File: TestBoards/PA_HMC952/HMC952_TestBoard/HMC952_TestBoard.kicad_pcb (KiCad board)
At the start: 2 copper layers, 60 x 45 mm, 31 parts, among them J1 SMA, J2 SMA, J3 VDD, J4 VGG, J5 VDET, J6 VDET, U1 HMC952ALP5GE

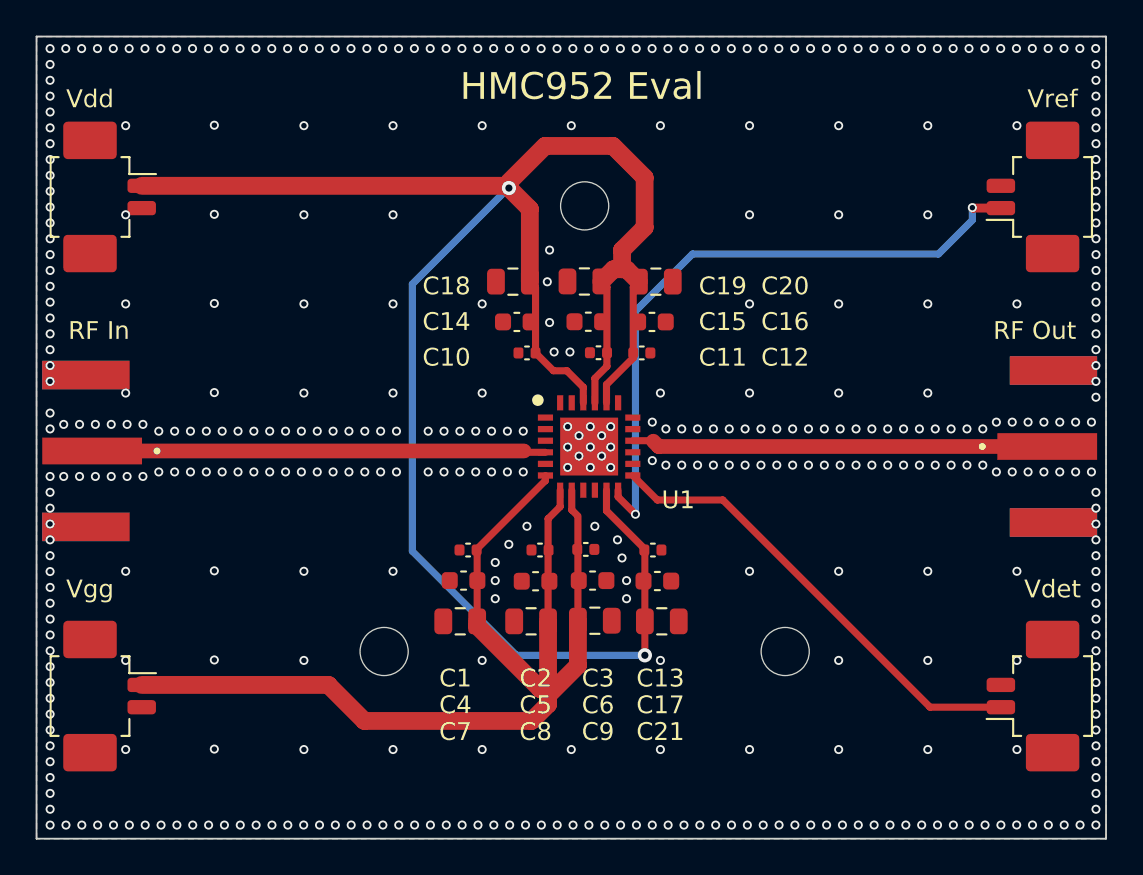
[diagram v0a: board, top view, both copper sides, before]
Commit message: XCOMMS RF Update
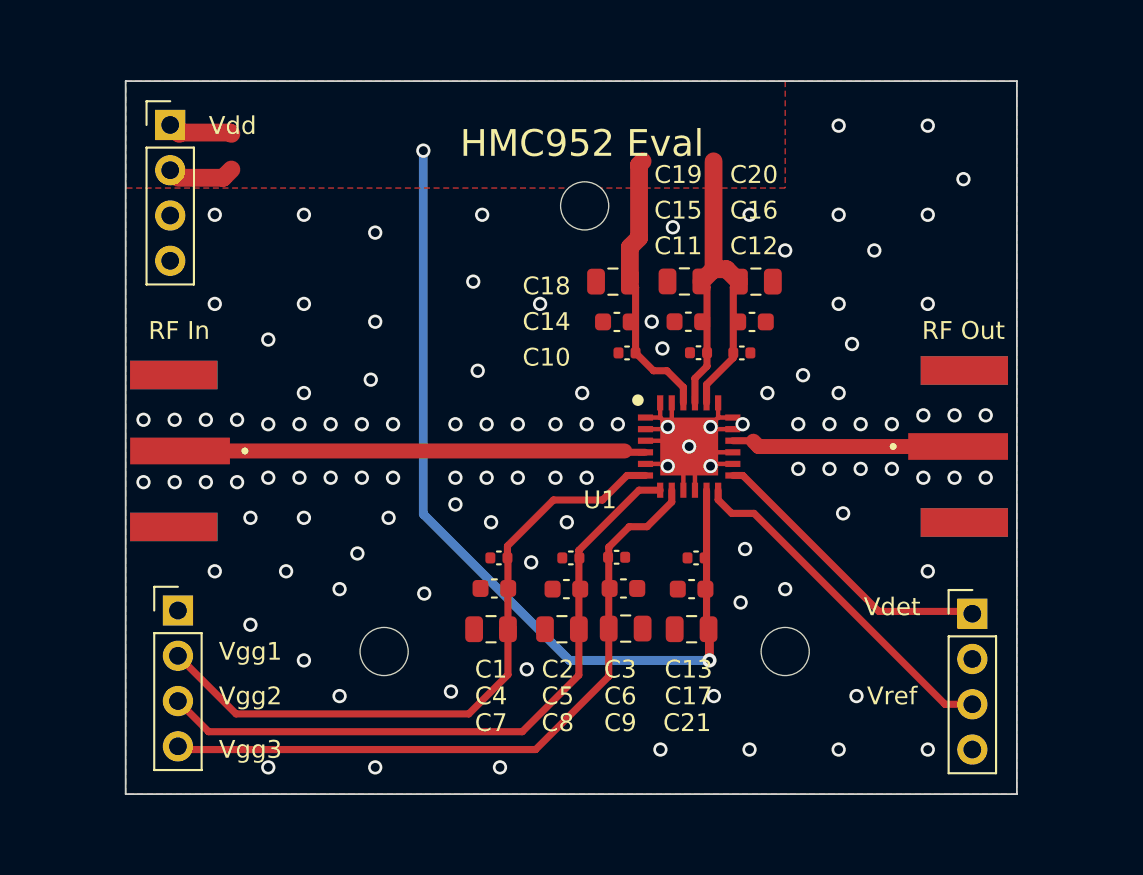
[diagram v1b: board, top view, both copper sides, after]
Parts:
- removed J6: VDET, Connector_Molex:Molex_PicoBlade_53261-0271_1x02-1MP_P1.25mm_Horizontal
- J3: value VDD -> Conn_01x04; footprint Connector_Molex:Molex_PicoBlade_53261-0271_1x02-1MP_P1.25mm_Horizontal -> Connector_PinHeader_2.54mm:PinHeader_1x04_P2.54mm_Vertical
- J4: value VGG -> Conn_01x04; footprint Connector_Molex:Molex_PicoBlade_53261-0271_1x02-1MP_P1.25mm_Horizontal -> Connector_PinHeader_2.54mm:PinHeader_1x04_P2.54mm_Vertical
- J5: value VDET -> Conn_01x04; footprint Connector_Molex:Molex_PicoBlade_53261-0271_1x02-1MP_P1.25mm_Horizontal -> Connector_PinHeader_2.54mm:PinHeader_1x04_P2.54mm_Vertical
- moved J4 6.53 mm to (113.9, 102.2), turned to 0 degrees
- moved J5 6.11 mm to (158.5, 102.4), turned to 0 degrees
- moved J3 5.69 mm to (113.5, 75.0), turned to 0 degrees
- moved C10 5.61 mm to (139.1, 87.8)
- moved C14 5.61 mm to (138.6, 86.0)
- moved C18 5.61 mm to (138.3, 83.8)
- moved U1 5.61 mm to (142.6, 93.0)
- moved C11 5.61 mm to (143.1, 87.7)
- moved C12 5.61 mm to (145.6, 87.8)
- moved C15 5.61 mm to (142.6, 86.0)
- moved C16 5.61 mm to (146.1, 86.0)
- moved C19 5.61 mm to (142.3, 83.7)
- moved C20 5.61 mm to (146.4, 83.8)
- moved J2 5.00 mm to (160.5, 93.0)
- moved J1 4.93 mm to (111.2, 93.2)
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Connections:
- C1 pad 2: /Vg_PA -> /Vg_PA1
- C2 pad 2: /Vg_PA -> /Vg_PA2
- C3 pad 2: /Vg_PA -> /Vg_PA3
- C4 pad 2: /Vg_PA -> /Vg_PA1
- C5 pad 2: /Vg_PA -> /Vg_PA2
- C6 pad 2: /Vg_PA -> /Vg_PA3
- C7 pad 2: /Vg_PA -> /Vg_PA1
- C8 pad 2: /Vg_PA -> /Vg_PA2
- C9 pad 2: /Vg_PA -> /Vg_PA3
- J3 pad 2: GND -> /Vd_PA
- J4 pad 1: /Vg_PA -> GND
- J4 pad 2: GND -> /Vg_PA1
- U1 pad 6: /Vg_PA -> /Vg_PA1
- U1 pad 7: /Vg_PA -> /Vg_PA2
- U1 pad 8: /Vg_PA -> /Vg_PA3
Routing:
- net /Vg_PA: track 64.0 -> 0.00 mm
- net /Vg_PA3: track 0.00 -> 38.4 mm
- net /Vg_PA1: track 0.00 -> 37.6 mm
- net /Vg_PA2: track 0.00 -> 37.5 mm
- net GND: track 0.00 -> 30.7 mm, vias 429 -> 111
- net /Vd_PA: track 115.4 -> 94.9 mm
- net /Vref: track 36.5 -> 19.6 mm, vias 2 -> 0
- net /RF_out: track 22.9 -> 12.8 mm
- net /Vdet: track 26.0 -> 16.6 mm
- net /RF_In: track 25.5 -> 26.2 mm
- added copper zone on F.Cu, net /Vd_PA
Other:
- board size 60 x 45 mm -> 50 x 40 mm
- board text added: "Vgg1"
- board text added: "Vgg2"
- board text added: "Vgg3"
- board text removed: "Vgg"
